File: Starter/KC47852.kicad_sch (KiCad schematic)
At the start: 49 parts, among them J1 Conn_01x09_Pin, J2 Speaker, J3 UART1, J4 Pot, J5 Joystick, J6 GND, J7 DACOUT, J8 Conn_01x05_Pin, SW1 UP, SW2 LEFT, SW3 DOWN, SW4 RGHT, U2 LP-MSPM0G3507, U3 MCP34119P, U4 HiLetGo_ST7735R, U5 ULN2003B, U6 TSOP31438

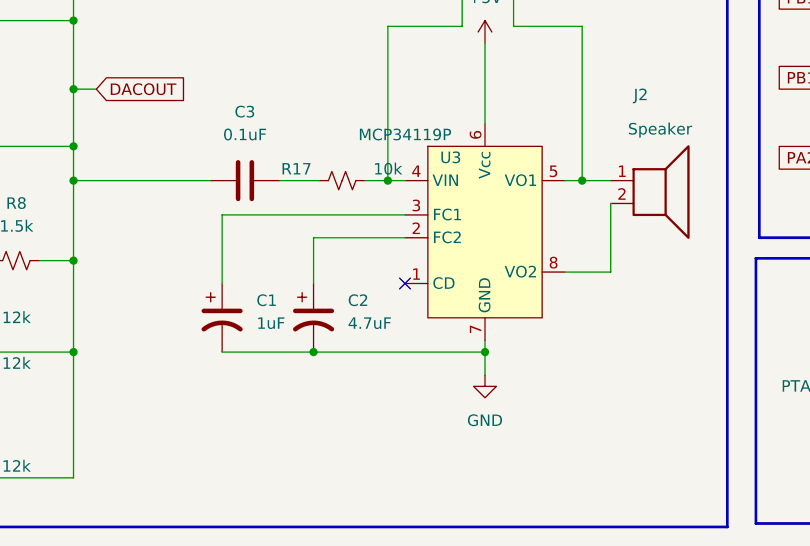
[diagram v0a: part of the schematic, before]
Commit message: bruh
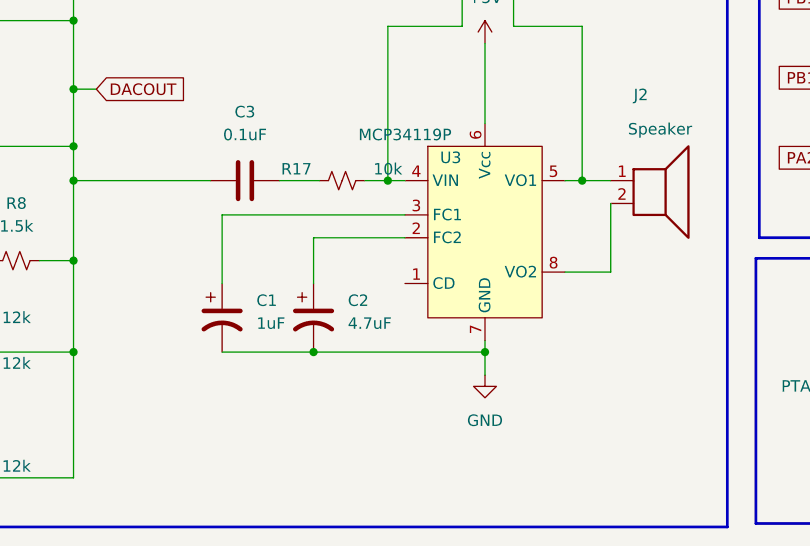
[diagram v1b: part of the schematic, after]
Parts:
- J1: footprint Connector_PinHeader_2.54mm:PinHeader_1x09_P2.54mm_Vertical -> (none)
- J8: footprint Connector_PinHeader_2.54mm:PinHeader_1x05_P2.54mm_Vertical -> (none)
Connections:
- no-connect marks 27 -> 26
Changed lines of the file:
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@@
 	)
 	(no_connect
-		(at 83.82 168.91)
-	)
-	(no_connect
 		(at 154.94 46.355)
 	)
@@
 			)
 		)
-		(property "Footprint" "Connector_PinHeader_2.54mm:PinHeader_1x05_P2.54mm_Vertical"
+		(property "Footprint" ""
 			(at 156.21 97.155 0)
 			(effects
@@
 			)
 		)
-		(property "Mouser #" ""
-			(at 156.21 97.155 0)
-			(effects
-				(font
-					(size 1.27 1.27)
-				)
-				(hide yes)
-			)
-		)
-		(property "Mouser Link" ""
-			(at 156.21 97.155 0)
-			(effects
-				(font
-					(size 1.27 1.27)
-				)
-				(hide yes)
-			)
-		)
-		(property "JLCPCB #" ""
-			(at 156.21 97.155 0)
-			(effects
-				(font
-					(size 1.27 1.27)
-				)
-				(hide yes)
-			)
-		)
 		(pin "1"
 		)
@@
 			)
 		)
-		(property "Footprint" "Connector_PinHeader_2.54mm:PinHeader_1x09_P2.54mm_Vertical"
+		(property "Footprint" ""
 			(at 130.81 104.775 0)
 			(effects
@@
 			(at 130.81 104.775 0)
 			(effects
-				(font
-					(size 1.27 1.27)
-				)
-				(hide yes)
-			)
-		)
-		(property "Mouser #" ""
-			(at 130.81 104.775 0)
-			(effects
-				(font
-					(size 1.27 1.27)
-				)
-				(hide yes)
-			)
-		)
-		(property "Mouser Link" ""
-			(at 130.81 104.775 0)
-			(effects
-				(font
-					(size 1.27 1.27)
-				)
-				(hide yes)
-			)
-		)
-		(property "JLCPCB #" ""
-			(at 130.81 104.775 0)
-			(effects

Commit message: Hai
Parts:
- J1: footprint (none) -> Connector_PinHeader_2.54mm:PinHeader_1x09_P2.54mm_Vertical
- J8: footprint (none) -> Connector_PinHeader_2.54mm:PinHeader_1x05_P2.54mm_Vertical
- U5: footprint ECE319H:DIP-16_W7.62mm -> Package_DIP:DIP-16_W7.62mm
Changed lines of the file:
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@@
 			)
 		)
-		(property "Footprint" ""
+		(property "Footprint" "Connector_PinHeader_2.54mm:PinHeader_1x05_P2.54mm_Vertical"
 			(at 156.21 97.155 0)
 			(effects
@@
 		)
 		(property "Description" "Generic connector, single row, 01x05, script generated"
+			(at 156.21 97.155 0)
+			(effects
+				(font
+					(size 1.27 1.27)
+				)
+				(hide yes)
+			)
+		)
+		(property "Mouser #" ""
+			(at 156.21 97.155 0)
+			(effects
+				(font
+					(size 1.27 1.27)
+				)
+				(hide yes)
+			)
+		)
+		(property "Mouser Link" ""
+			(at 156.21 97.155 0)
+			(effects
+				(font
+					(size 1.27 1.27)
+				)
+				(hide yes)
+			)
+		)
+		(property "JLCPCB #" ""
 			(at 156.21 97.155 0)
 			(effects
@@
 			)
 		)
-		(property "Footprint" ""
+		(property "Footprint" "Connector_PinHeader_2.54mm:PinHeader_1x09_P2.54mm_Vertical"
 			(at 130.81 104.775 0)
 			(effects
@@
 		)
 		(property "Description" "Generic connector, single row, 01x09, script generated"
+			(at 130.81 104.775 0)
+			(effects
+				(font
+					(size 1.27 1.27)
+				)
+				(hide yes)
+			)
+		)
+		(property "Mouser #" ""
+			(at 130.81 104.775 0)
+			(effects
+				(font
+					(size 1.27 1.27)
+				)
+				(hide yes)
+			)
+		)
+		(property "Mouser Link" ""
+			(at 130.81 104.775 0)
+			(effects
+				(font
+					(size 1.27 1.27)
+				)
+				(hide yes)
+			)
+		)
+		(property "JLCPCB #" ""
 			(at 130.81 104.775 0)
 			(effects
@@
 			)
 		)
-		(property "Footprint" "ECE319H:DIP-16_W7.62mm"
+		(property "Footprint" "Package_DIP:DIP-16_W7.62mm"
 			(at 196.85 48.26 0)
 			(effects
